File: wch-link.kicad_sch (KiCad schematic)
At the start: 31 parts, among them J1 USB2.0_C_v3, J2 SWD-Debugger_Side-10Pin, SW1 SW_Push, U1 AMS1117-3.3, U2 CH32V305FBP6, Y1 12M

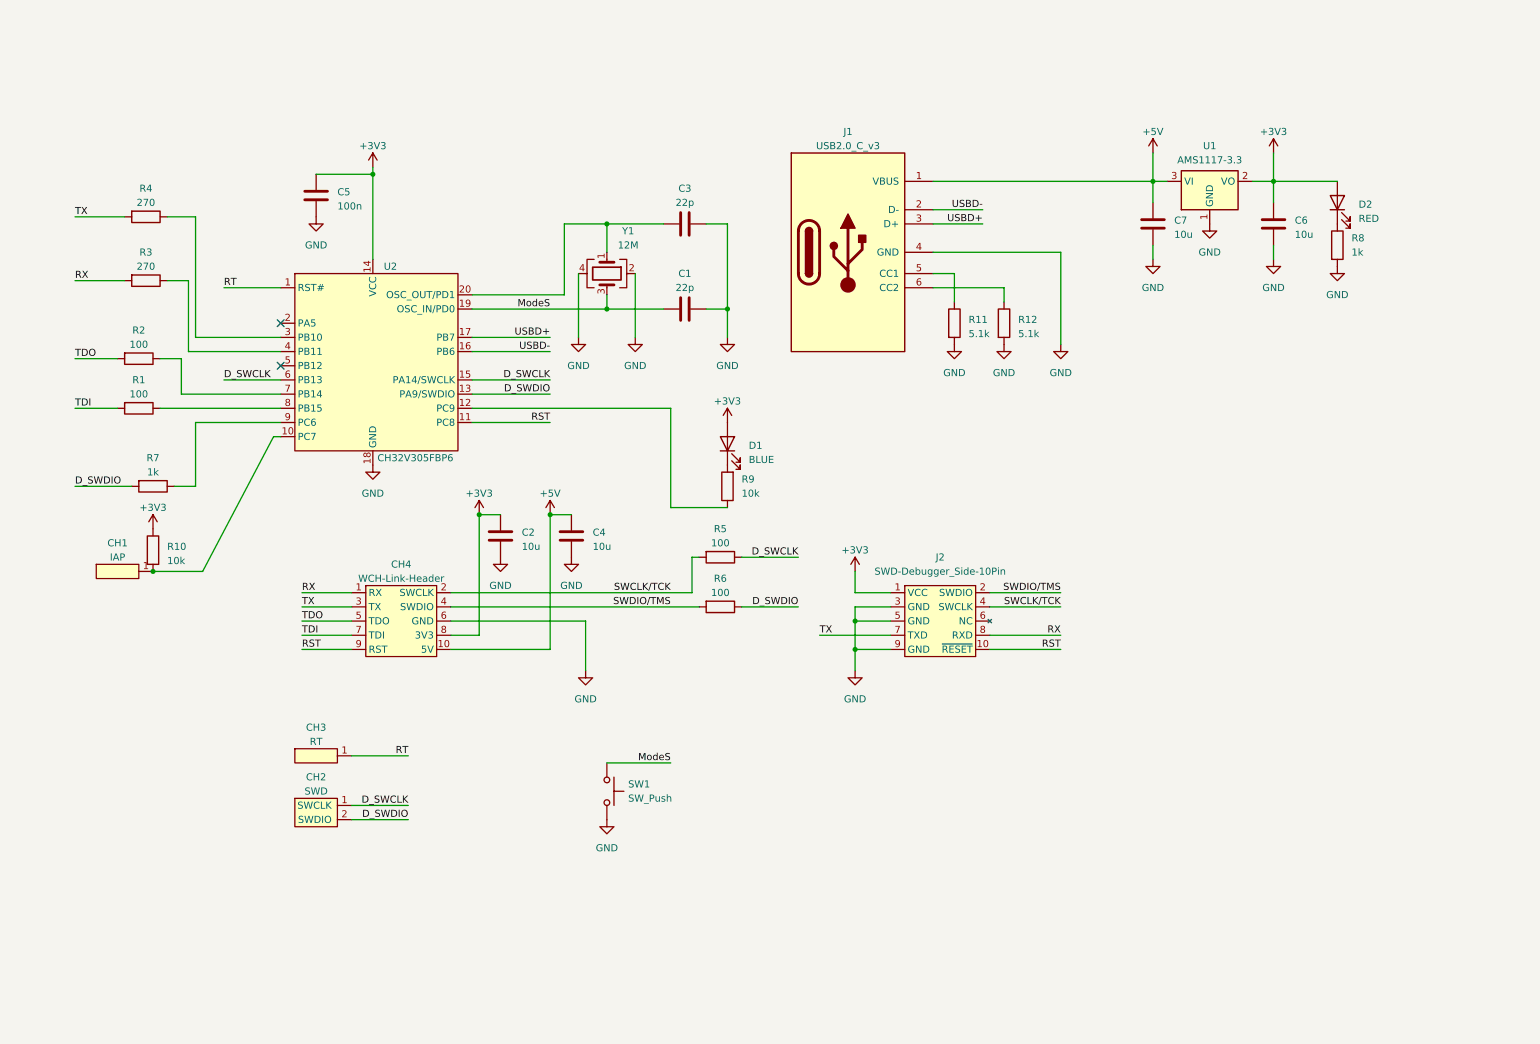
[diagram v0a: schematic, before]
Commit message: v1.1.1
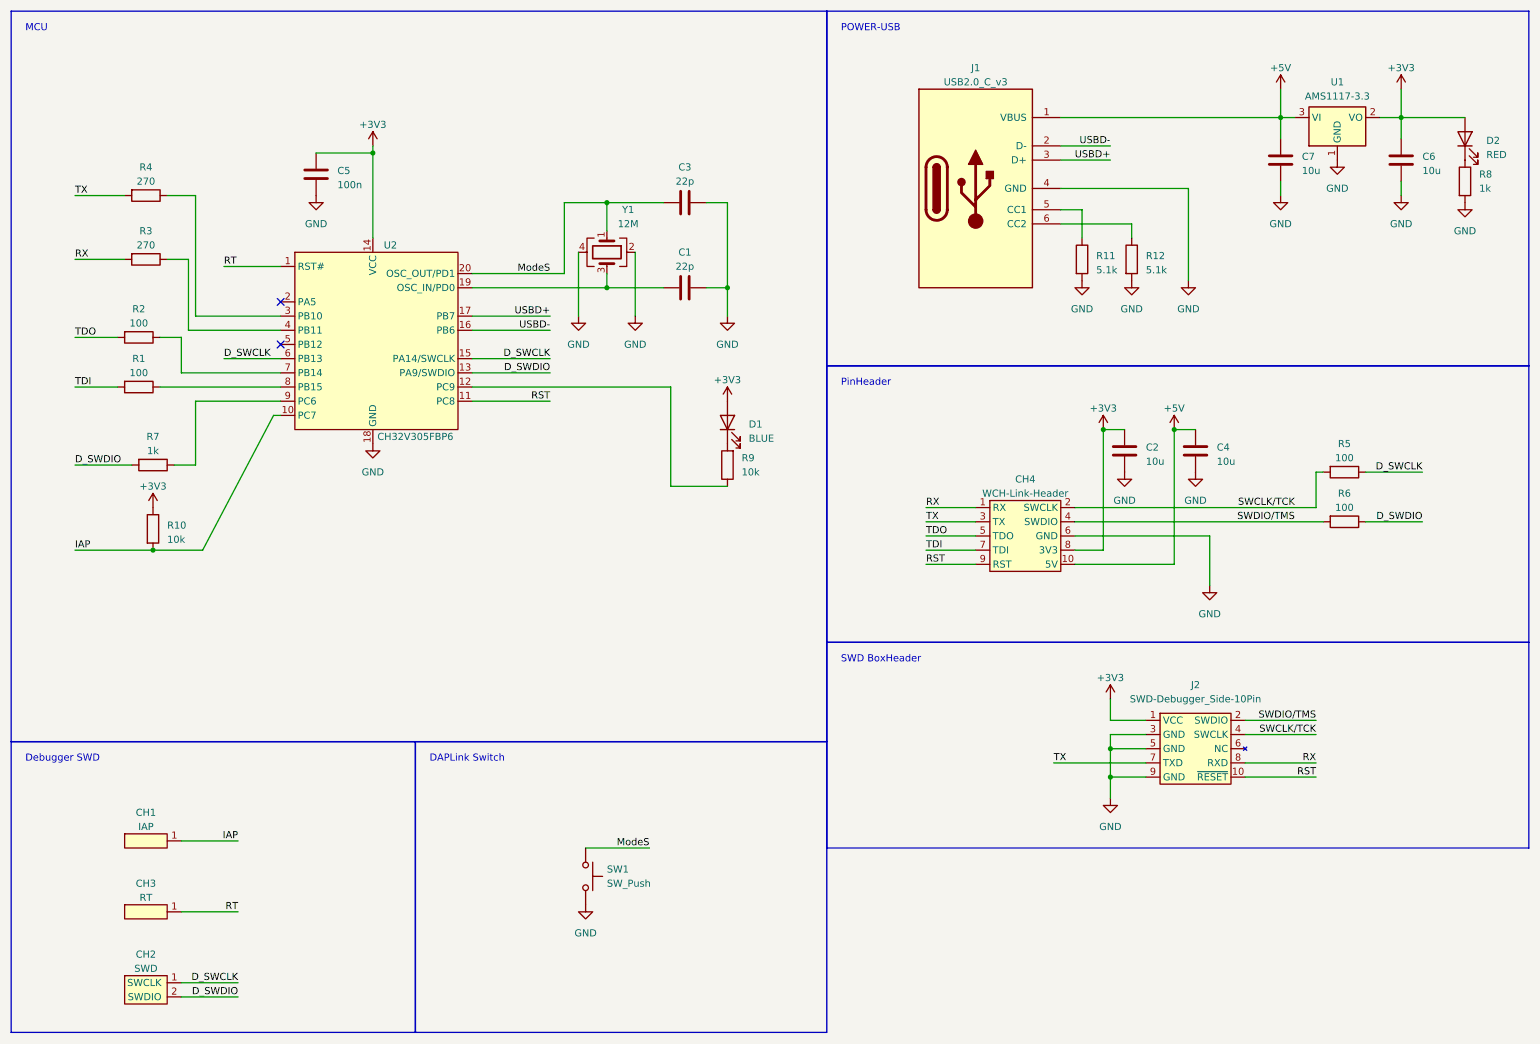
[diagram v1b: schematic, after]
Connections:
- net ModeS: now also C3.2, U2.20 (OSC_OUT/PD1), Y1.1; no longer C1.2, U2.19 (OSC_IN/PD0), Y1.3
- net IAP: now reaches CH1.1, R10.2, U2.10 (PC7)
- new net: C1.2, U2.19 (OSC_IN/PD0), Y1.3
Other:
- note added: "DAPLink Switch"
- note added: "Debugger SWD"
- note added: "MCU"
- note added: "POWER-USB"
- note added: "PinHeader"
- note added: "SWD BoxHeader"
- moved on the sheet: C1, C2, C3, C4, C5, C6, C7, CH1, CH2, CH3, CH4, D1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
